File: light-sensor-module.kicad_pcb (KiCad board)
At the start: 2 copper layers, 36.8 x 29.2 mm, 18 parts, among them P1 MOLEX_01X06, P2 HEADER_01X06, P3 TERM_01X02, U1 STR05, U2 VEML6030, U3 BH1750

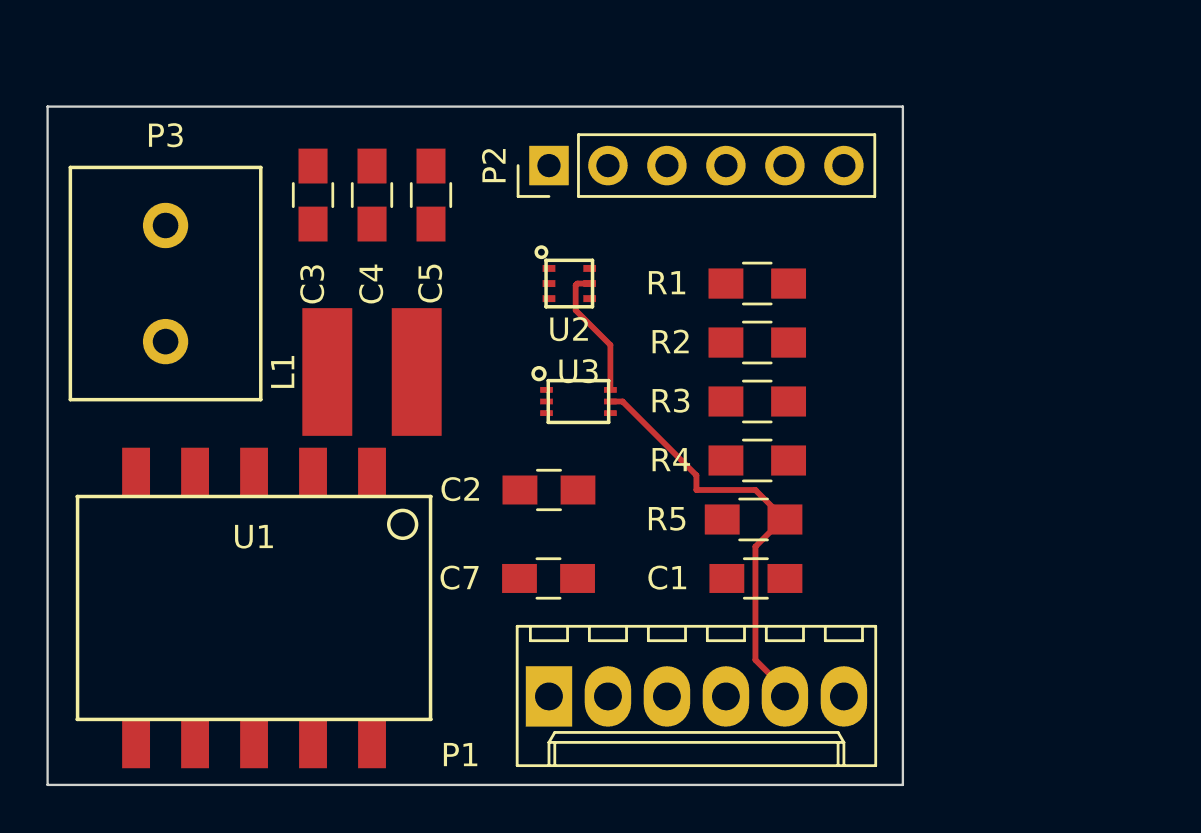
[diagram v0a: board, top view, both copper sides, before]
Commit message: Complete PCB design
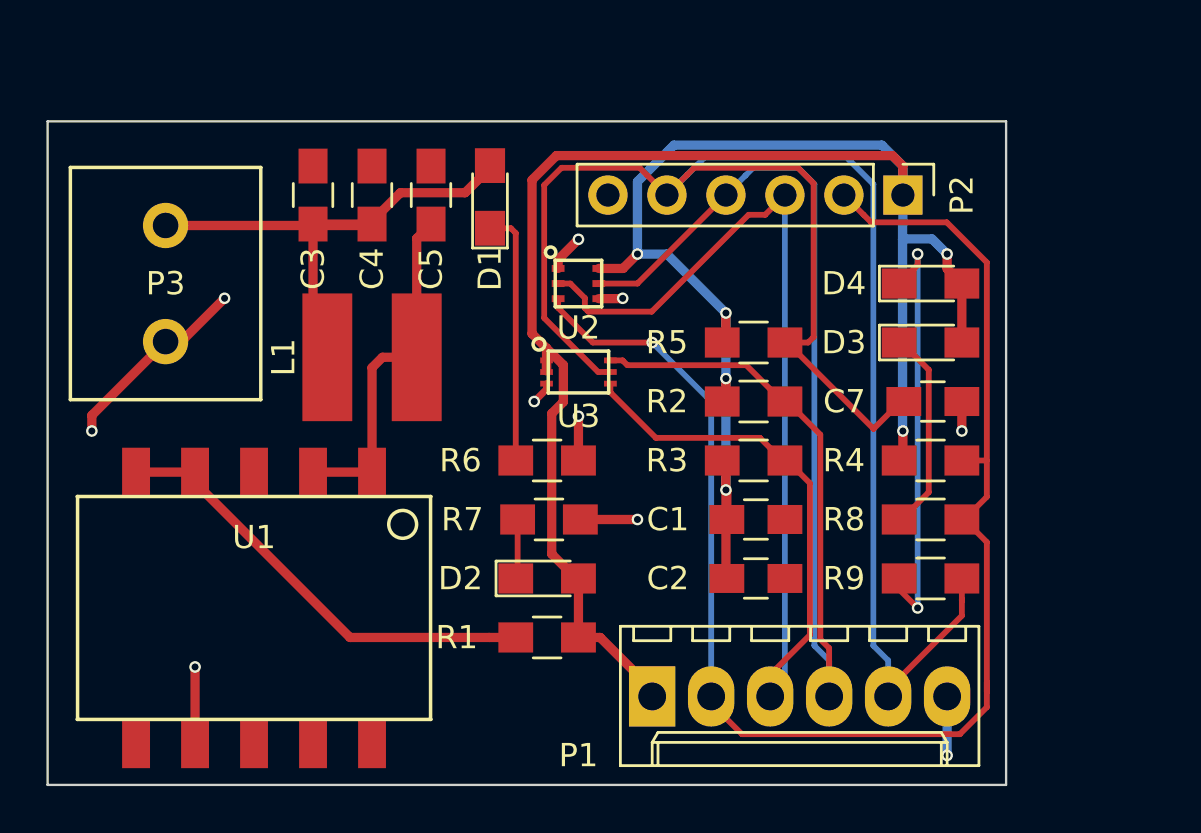
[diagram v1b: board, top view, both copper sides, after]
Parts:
- added D1: LED, LEDs:LED_0805_HandSoldering, F.Cu at (130.8, 97.9)
- added D2: LED, LEDs:LED_0805_HandSoldering, F.Cu at (133.3, 114.3)
- added D3: LED, LEDs:LED_0805_HandSoldering, F.Cu at (149.8, 104.1)
- added D4: LED, LEDs:LED_0805_HandSoldering, F.Cu at (149.8, 101.6)
- added R6: 470R, Resistors_SMD:R_0805_HandSoldering, F.Cu at (133.3, 109.2)
- added R7: 470R, Resistors_SMD:R_0805_HandSoldering, F.Cu at (133.3, 111.8)
- added R8: 470R, Resistors_SMD:R_0805_HandSoldering, F.Cu at (149.8, 111.8)
- added R9: 470R, Resistors_SMD:R_0805_HandSoldering, F.Cu at (149.8, 114.3)
- moved C7 18.2 mm to (149.9, 106.7)
- moved R1 17.7 mm to (133.3, 116.8), turned to 180 degrees
- moved P2 15.3 mm to (148.6, 97.8), turned to 270 degrees
- moved C2 9.69 mm to (142.3, 114.3)
- moved R5 7.62 mm to (142.2, 104.1)
- moved R4 7.46 mm to (149.8, 109.2)
- moved P1 4.44 mm to (137.8, 119.4)
- moved R2 2.55 mm to (142.2, 106.7)
- moved R3 2.55 mm to (142.2, 109.2)
- moved C1 2.54 mm to (142.3, 111.8)
- moved U3 1.27 mm to (134.6, 105.4)
- moved L1 0.63 mm to (125.7, 104.8)
- moved U2 0.40 mm to (134.6, 101.6)
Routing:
- net VCC+3: track 0.00 -> 102.5 mm, vias 0 -> 6
- net INT: track 0.00 -> 63.6 mm, vias 0 -> 1
- net DVI: track 18.7 -> 76.6 mm
- net SDA: track 0.00 -> 54.9 mm
- net SCL: track 5.76 -> 55.8 mm
- net VIN+12: track 0.00 -> 23.7 mm
- net GNDREF: track 0.00 -> 23.6 mm, vias 0 -> 10
- net VREG+3: track 0.00 -> 19.6 mm
- net Net-(D4-Pad1): track 0.00 -> 19.0 mm, vias 0 -> 2
- net Net-(C5-Pad1): track 0.00 -> 15.1 mm
- net Net-(D1-Pad1): track 0.00 -> 11.0 mm
- net Net-(D3-Pad1): track 0.00 -> 8.79 mm
- net Net-(D2-Pad1): track 0.00 -> 2.57 mm
- added copper zone on B.Cu, net GNDREF
- added copper zone on F.Cu, net GNDREF
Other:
- board size 36.8 x 29.2 mm -> 41.3 x 28.6 mm
- net class Default: via_dia 0.6 -> 0.5; via_drill 0.4 -> 0.3

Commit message: Add Gerbers, PDFs and Drill File
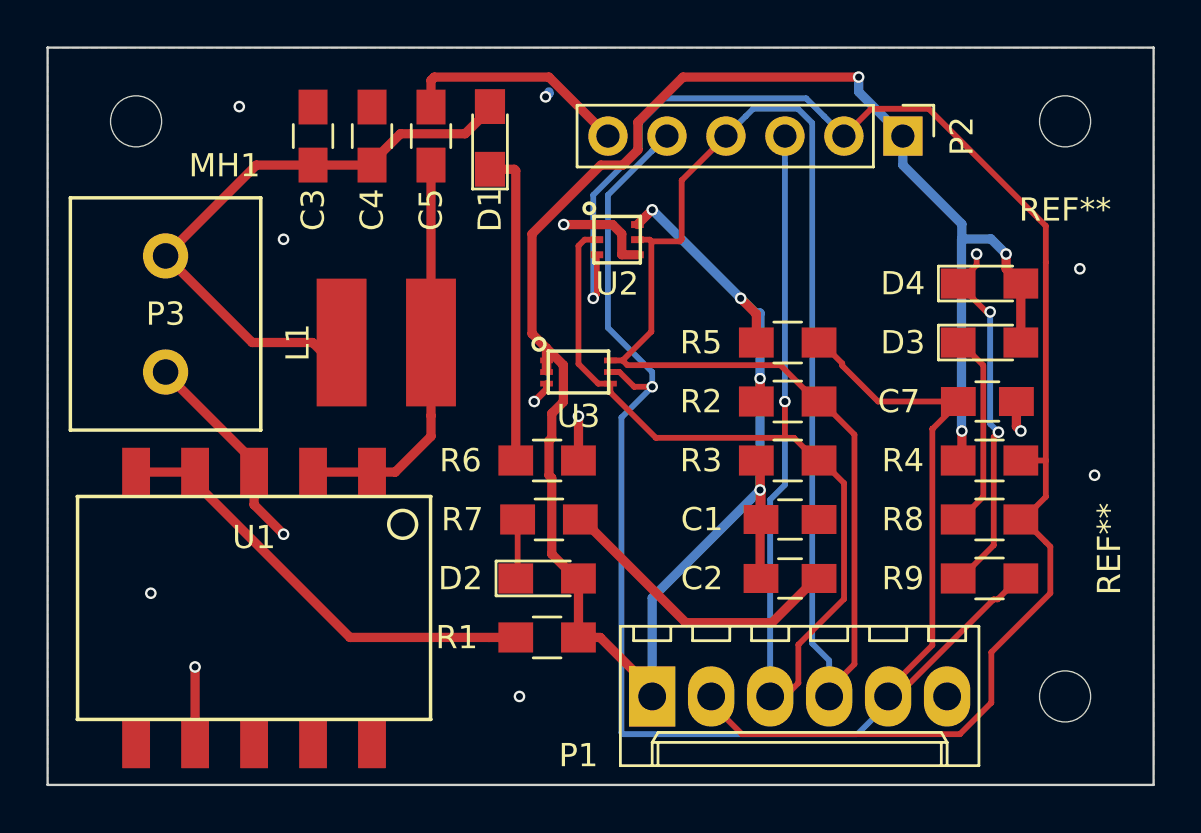
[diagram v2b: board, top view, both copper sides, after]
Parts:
- added MH1: MountingHole_2.2mm_M2, Mounting_Holes:MountingHole_2.2mm_M2, F.Cu at (115.6, 94.6)
- added REF**: MountingHole_2.2mm_M2, Mounting_Holes:MountingHole_2.2mm_M2, F.Cu at (155.6, 119.4)
- added REF**: MountingHole_2.2mm_M2, Mounting_Holes:MountingHole_2.2mm_M2, F.Cu at (155.6, 94.6)
- moved C3 2.54 mm to (123.2, 95.2)
- moved C4 2.54 mm to (125.7, 95.2)
- moved C5 2.54 mm to (128.3, 95.2)
- moved D1 2.54 mm to (130.8, 95.3)
- moved P2 2.54 mm to (148.6, 95.2)
- moved D3 2.54 mm to (152.3, 104.1)
- moved D4 2.54 mm to (152.3, 101.6)
- moved R4 2.54 mm to (152.3, 109.2)
- moved R8 2.54 mm to (152.3, 111.8)
- moved R9 2.54 mm to (152.3, 114.3)
- moved U2 2.52 mm to (136.3, 99.7)
- moved C7 2.35 mm to (152.2, 106.7)
- moved C1 1.47 mm to (143.7, 111.8)
- moved C2 1.47 mm to (143.7, 114.3)
- moved R2 1.47 mm to (143.6, 106.7)
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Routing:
- net GNDREF: track 23.6 -> 43.7 mm, vias 10 -> 6
- net SCL: track 55.8 -> 65.9 mm
- net INT: track 63.6 -> 68.7 mm
- net DVI: track 76.6 -> 72.6 mm, vias 0 -> 1
- net Net-(D1-Pad1): track 11.0 -> 13.6 mm
- net Net-(C5-Pad1): track 15.1 -> 17.4 mm
- net Net-(D4-Pad1): track 19.0 -> 16.8 mm, vias 2 -> 3
- net VIN+12: track 23.7 -> 25.6 mm
- net SDA: track 54.9 -> 56.6 mm, vias 0 -> 1
- net (no net): track 0.00 -> 0.28 mm, vias 0 -> 7
- net VCC+3: vias 6 -> 7
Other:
- board size 41.3 x 28.6 mm -> 47.6 x 31.8 mm
